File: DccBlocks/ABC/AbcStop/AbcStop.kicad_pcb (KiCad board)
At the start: 2 copper layers, 51 x 18 mm, 8 parts, among them J1 SCREW, J2 43650-0200

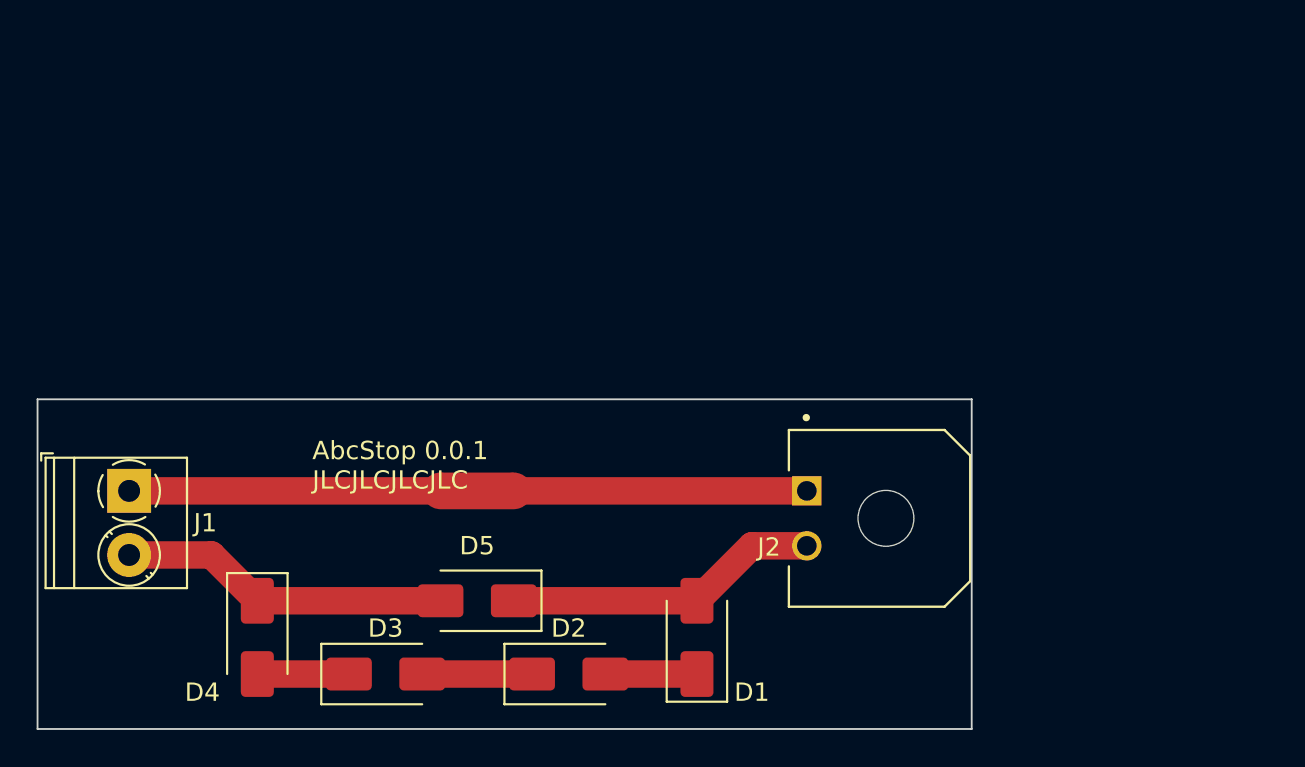
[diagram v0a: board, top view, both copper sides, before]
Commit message: AbcStop
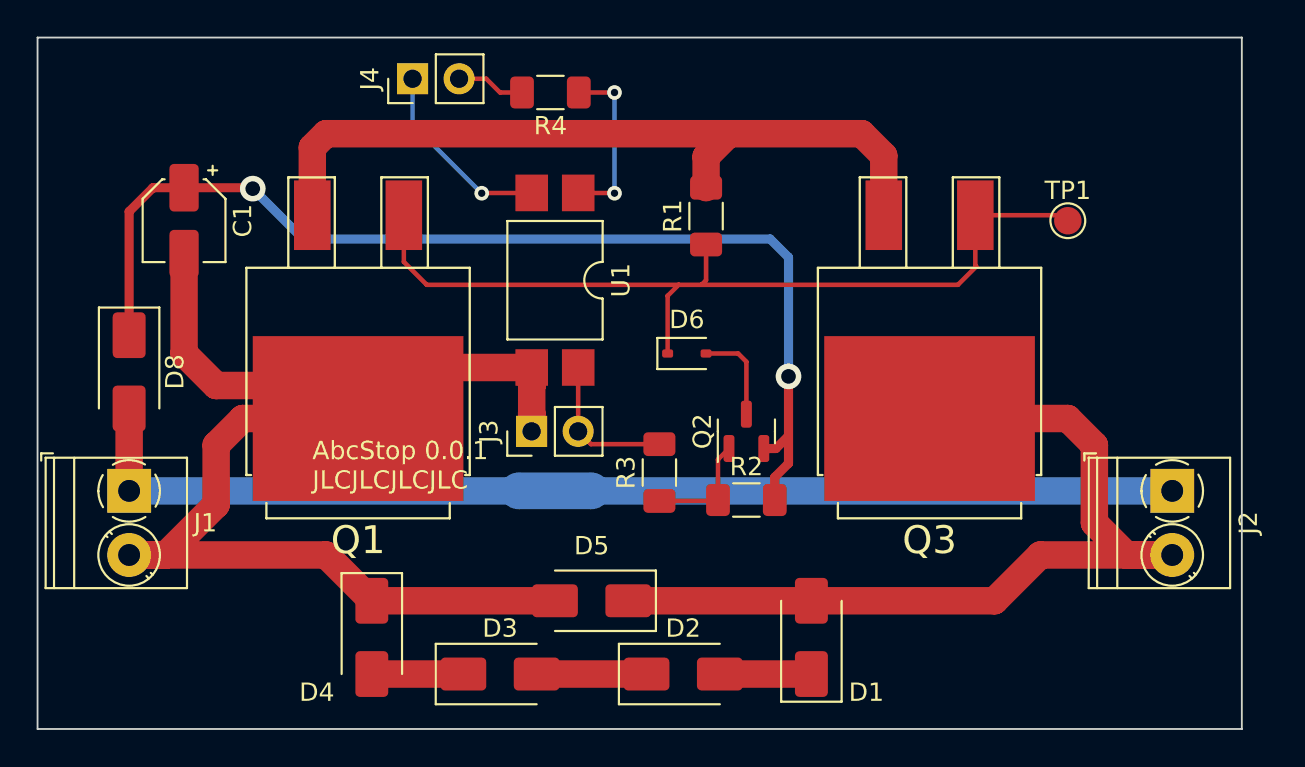
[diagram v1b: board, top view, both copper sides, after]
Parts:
- added C1: 4.7uF, Capacitor_SMD:CP_Elec_4x5.4, F.Cu at (66.0, 45.2)
- added D6: 1N4148, Diode_SMD:D_SOD-323, F.Cu at (93.5, 52.5)
- added D8: ES1G+, Diode_SMD:D_SMA, F.Cu at (63.0, 53.5)
- added J3: Conn_01x02, Connector_PinHeader_2.54mm:PinHeader_1x02_P2.54mm_Vertical, F.Cu at (85.0, 56.8)
- added J4: Conn_01x02, Connector_PinHeader_2.54mm:PinHeader_1x02_P2.54mm_Vertical, F.Cu at (78.5, 37.5)
- added Q1: PSMN022, DigitalTrains:sot404, F.Cu at (75.5, 50.5)
- added Q2: Q_PMOS_GSD, Package_TO_SOT_SMD:SOT-23, F.Cu at (96.7, 56.8)
- added Q3: PSMN022, DigitalTrains:sot404, F.Cu at (106.7, 50.5)
- added R1: 1K, Resistor_SMD:R_1206_3216Metric_Pad1.30x1.75mm_HandSolder, F.Cu at (94.5, 45.0)
- added R2: 3K, Resistor_SMD:R_1206_3216Metric_Pad1.30x1.75mm_HandSolder, F.Cu at (96.7, 60.5)
- added R3: 1K, Resistor_SMD:R_1206_3216Metric_Pad1.30x1.75mm_HandSolder, F.Cu at (92.0, 59.0)
- added R4: 3K, Resistor_SMD:R_1206_3216Metric_Pad1.30x1.75mm_HandSolder, F.Cu at (86.0, 38.2)
- added TP1: TestPoint, TestPoint:TestPoint_Pad_D1.5mm, F.Cu at (114.2, 45.2)
- added U1: VO615A, Package_DIP:SMDIP-4_W9.53mm, F.Cu at (86.2, 48.5)
- J2: value 43650-0200 -> SCREW; footprint DigitalTrains:MOLEX_436500200 -> TerminalBlock_Phoenix:TerminalBlock_Phoenix_PT-1,5-2-3.5-H_1x02_P3.50mm_Horizontal
- NT1: moved to B.Cu
- moved J2 16.1 mm to (120.0, 60.0), turned to -90 degrees
- moved D1 6.25 mm to (100.2, 68.0)
- moved D2 6.25 mm to (93.2, 70.0)
- moved D3 6.25 mm to (83.2, 70.0)
- moved D4 6.25 mm to (76.2, 68.0)
- moved D5 6.25 mm to (88.2, 66.0)
- moved NT1 4.25 mm to (86.2, 60.0)
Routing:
- net /High_Right: track 0.00 -> 60.4 mm, vias 0 -> 2
- net /Right_IN: track 18.0 -> 74.6 mm
- net Net-(D6-K): track 0.00 -> 49.2 mm
- net /Right_1: track 0.00 -> 42.4 mm
- net /Right_OUT: track 17.2 -> 49.6 mm
- net /Left_OUT: track 16.0 -> 31.7 mm
- net /enGnd: track 0.00 -> 10.5 mm, vias 0 -> 1
- net Net-(R4-Pad1): track 0.00 -> 9.44 mm, vias 0 -> 2
- net /Left_IN: track 17.0 -> 25.5 mm
- net Net-(J3-Pin_2): track 0.00 -> 8.21 mm
- net /GRight: track 0.00 -> 6.28 mm
- net Net-(D6-A): track 0.00 -> 5.25 mm
- net /en: track 0.00 -> 3.75 mm
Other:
- board size 51 x 18 mm -> 65.8 x 37.8 mm
